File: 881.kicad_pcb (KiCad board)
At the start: 2 copper layers, 38 x 105 mm, 0 parts

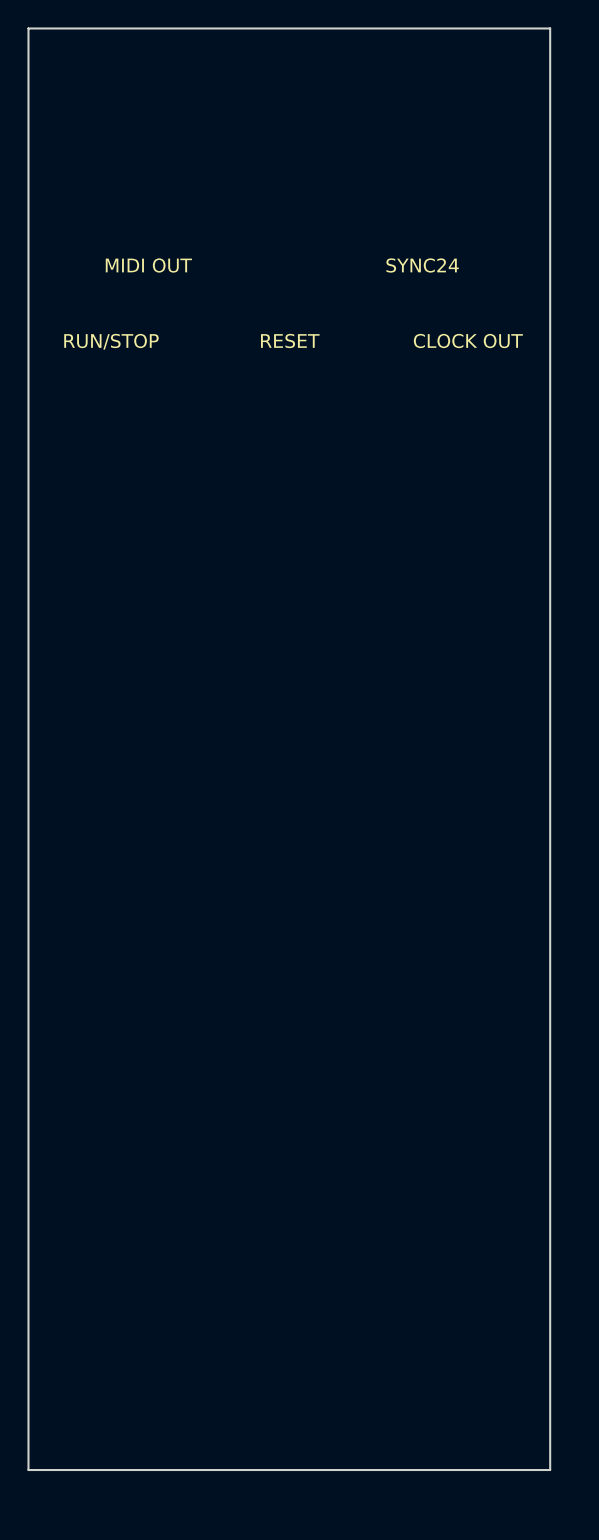
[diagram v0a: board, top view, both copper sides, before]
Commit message: first route
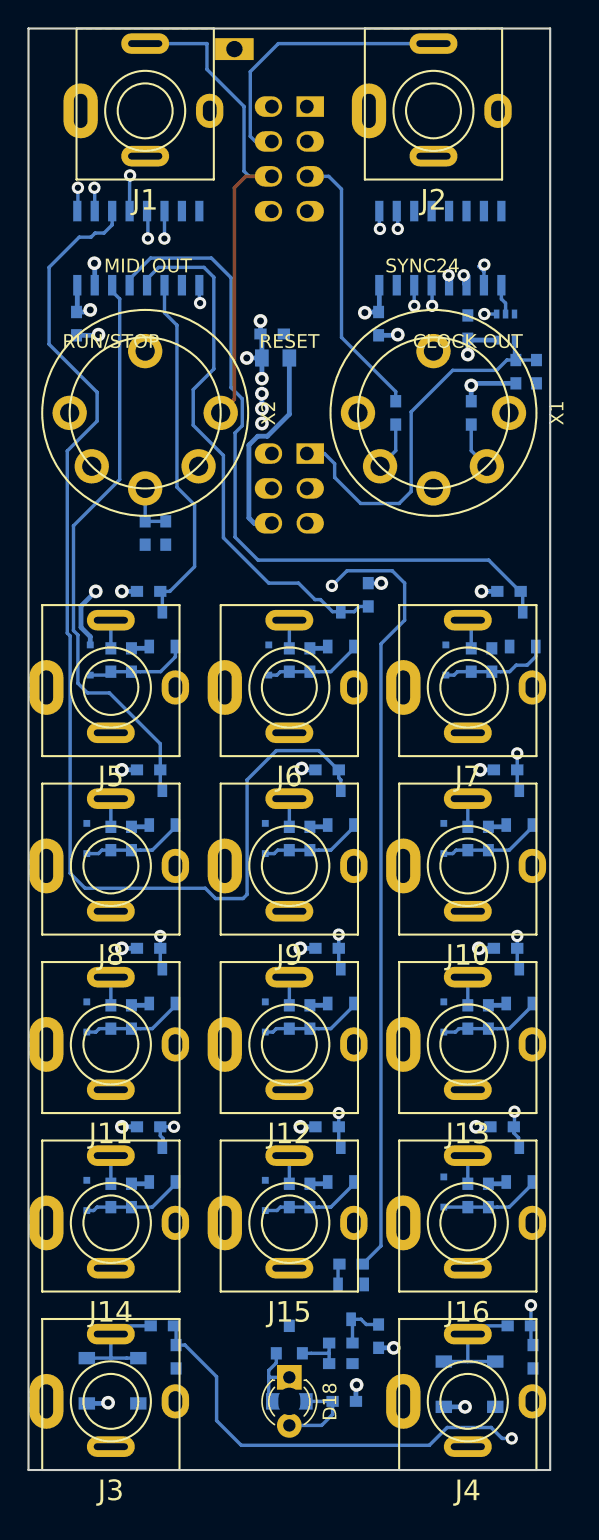
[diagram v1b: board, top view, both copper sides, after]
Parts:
- added C1: 0.01µ, MyModules:SM0603-C-MURATA, B.Cu at (121.5, 91.8)
- added C15: 1µ, Capacitors_SMD:C_0805, B.Cu at (129.5, 79.0)
- added C19: 0.1µ, MyModules:SM0603-C-MURATA, B.Cu at (129.2, 77.2)
- added C2: 0.1µ, MyModules:SM0603-C-MURATA, B.Cu at (115.0, 76.5)
- added C20: 0.1µ, MyModules:SM0603-C-MURATA, B.Cu at (143.5, 76.8)
- added C3: 0.1µ, MyModules:SM0603-C-MURATA, B.Cu at (137.0, 76.5)
- added C4: 1n, MyModules:SM0603-C-MURATA, B.Cu at (134.2, 152.2)
- added D1: B5819W, Diodes_SMD:D_SOD-123, B.Cu at (115.8, 153.5)
- added D10: 1N4148, Diodes_SMD:D_SOD-323F, B.Cu at (141.8, 114.0)
- added D11: 1N4148, Diodes_SMD:D_SOD-323F, B.Cu at (115.8, 127.0)
- added D12: 1N4148, Diodes_SMD:D_SOD-323F, B.Cu at (128.8, 127.0)
- added D13: 1N4148, Diodes_SMD:D_SOD-323F, B.Cu at (141.8, 127.0)
- added D14: 1N4148, Diodes_SMD:D_SOD-323F, B.Cu at (115.8, 140.0)
- added D15: 1N4148, Diodes_SMD:D_SOD-323F, B.Cu at (128.8, 140.0)
- added D16: 1N4148, Diodes_SMD:D_SOD-323F, B.Cu at (141.8, 139.8)
- added D17: LED, LEDs:LED_0805, B.Cu at (130.5, 155.0)
- added D18: LED, LEDs:LED_D3.0mm, F.Cu at (130.5, 153.8)
- added D2: B5819W, Diodes_SMD:D_SOD-123, B.Cu at (119.5, 153.5)
- added D3: B5819W, Diodes_SMD:D_SOD-123, B.Cu at (141.8, 153.8)
- added D4: B5819W, Diodes_SMD:D_SOD-123, B.Cu at (145.5, 153.8)
- added D5: 1N4148, Diodes_SMD:D_SOD-323F, B.Cu at (116.0, 101.0)
- added D6: 1N4148, Diodes_SMD:D_SOD-323F, B.Cu at (129.0, 101.0)
- added D7: 1N4148, Diodes_SMD:D_SOD-323F, B.Cu at (141.9, 101.0)
- added D8: 1N4148, Diodes_SMD:D_SOD-323F, B.Cu at (115.8, 114.0)
- added D9: 1N4148, Diodes_SMD:D_SOD-323F, B.Cu at (128.8, 114.0)
- added ISP1: CONN_02X03, w_conn_strip:vasch_strip_3x2, B.Cu at (130.5, 88.5)
- added J1: RUN/STOP, MyModules:PJ-301B-JACK-SLOTS, F.Cu at (120.0, 61.0)
- added J10: RS IN, MyModules:PJ-301B-JACK-SLOTS, F.Cu at (143.5, 116.0)
- added J11: CP IN, MyModules:PJ-301B-JACK-SLOTS, F.Cu at (117.5, 129.0)
- added J12: MA IN, MyModules:PJ-301B-JACK-SLOTS, F.Cu at (130.5, 129.0)
- added J13: CB IN, MyModules:PJ-301B-JACK-SLOTS, F.Cu at (143.5, 129.0)
- added J14: CY IN, MyModules:PJ-301B-JACK-SLOTS, F.Cu at (117.5, 142.0)
- added J15: OH IN, MyModules:PJ-301B-JACK-SLOTS, F.Cu at (130.5, 142.0)
- added J16: CH IN, MyModules:PJ-301B-JACK-SLOTS, F.Cu at (143.5, 142.0)
- added J2: SYNC24 CLK, MyModules:PJ-301B-JACK-SLOTS, F.Cu at (141.0, 61.0)
- added J3: ASSIGN 1, MyModules:PJ-301B-JACK-SLOTS, F.Cu at (117.5, 155.0)
- added J4: ASSIGN 2, MyModules:PJ-301B-JACK-SLOTS, F.Cu at (143.5, 155.0)
- added J5: BD IN, MyModules:PJ-301B-JACK-SLOTS, F.Cu at (117.5, 103.0)
- added J6: SD IN, MyModules:PJ-301B-JACK-SLOTS, F.Cu at (130.5, 103.0)
- added J7: LT IN, MyModules:PJ-301B-JACK-SLOTS, F.Cu at (143.5, 103.0)
- added J8: MT IN, MyModules:PJ-301B-JACK-SLOTS, F.Cu at (117.5, 116.0)
- added J9: HT IN, MyModules:PJ-301B-JACK-SLOTS, F.Cu at (130.5, 116.0)
- added P1: CONN_02X03, w_conn_strip:vasch_strip_4x2, B.Cu at (130.5, 64.5)
- added Q1: MMBT3904, MyModules:SOT23-132-JRL, B.Cu at (121.2, 98.8)
- added Q10: MMBT3904, MyModules:SOT23-132-JRL, B.Cu at (121.2, 137.8)
- added Q11: MMBT3904, MyModules:SOT23-132-JRL, B.Cu at (134.2, 137.8)
- added Q12: MMBT3904, MyModules:SOT23-132-JRL, B.Cu at (147.2, 137.8)
- added Q13: MMBT3904, MyModules:SOT23-132-JRL, B.Cu at (135.0, 147.8)
- added Q14: MMBT3906, SOT-23, B.Cu at (130.5, 150.5)
- added Q2: MMBT3904, MyModules:SOT23-132-JRL, B.Cu at (134.2, 98.8)
- added Q3: MMBT3904, MyModules:SOT23-132-JRL, B.Cu at (147.5, 98.8)
- added Q4: MMBT3904, MyModules:SOT23-132-JRL, B.Cu at (121.2, 111.8)
- added Q5: MMBT3904, MyModules:SOT23-132-JRL, B.Cu at (134.2, 111.8)
- added Q6: MMBT3904, MyModules:SOT23-132-JRL, B.Cu at (147.2, 111.8)
- added Q7: MMBT3904, MyModules:SOT23-132-JRL, B.Cu at (121.2, 124.8)
- added Q8: MMBT3904, MyModules:SOT23-132-JRL, B.Cu at (134.2, 124.8)
- added Q9: MMBT3904, MyModules:SOT23-132-JRL, B.Cu at (147.2, 124.8)
- added R1: 220, MyModules:SM0603-R-YAGEO, B.Cu at (138.2, 83.0)
- added R10: 100K, MyModules:SM0603-R-YAGEO, B.Cu at (119.0, 101.0)
- added R11: 100K, MyModules:SM0603-R-YAGEO, B.Cu at (132.0, 101.0)
- added R12: 100K, MyModules:SM0603-R-YAGEO, B.Cu at (145.2, 101.0)
- added R13: 100K, MyModules:SM0603-R-YAGEO, B.Cu at (119.0, 114.0)
- added R14: 10K, MyModules:SM0603-R-YAGEO, B.Cu at (120.2, 96.0)
- added R15: 10K, MyModules:SM0603-R-YAGEO, B.Cu at (136.2, 96.2)
- added R16: 10K, MyModules:SM0603-R-YAGEO, B.Cu at (146.5, 96.0)
- added R17: 10K, MyModules:SM0603-R-YAGEO, B.Cu at (120.2, 109.0)
- added R18: 100K, MyModules:SM0603-R-YAGEO, B.Cu at (130.5, 114.0)
- added R19: 100K, MyModules:SM0603-R-YAGEO, B.Cu at (143.5, 114.0)
- added R2: 22, MyModules:SM0603-R-YAGEO, B.Cu at (120.0, 91.8)
- added R20: 100K, MyModules:SM0603-R-YAGEO, B.Cu at (117.5, 127.0)
- added R21: 100K, MyModules:SM0603-R-YAGEO, B.Cu at (130.5, 127.0)
- added R22: 100K, MyModules:SM0603-R-YAGEO, B.Cu at (132.0, 114.0)
- added R23: 100K, MyModules:SM0603-R-YAGEO, B.Cu at (145.0, 114.0)
- added R24: 100K, MyModules:SM0603-R-YAGEO, B.Cu at (119.0, 127.0)
- added R25: 100K, MyModules:SM0603-R-YAGEO, B.Cu at (132.0, 127.0)
- added R26: 10K, MyModules:SM0603-R-YAGEO, B.Cu at (133.2, 109.0)
- added R27: 10K, MyModules:SM0603-R-YAGEO, B.Cu at (146.2, 109.0)
- added R28: 10K, MyModules:SM0603-R-YAGEO, B.Cu at (120.2, 122.0)
- added R29: 10K, MyModules:SM0603-R-YAGEO, B.Cu at (133.2, 122.0)
- added R3: 220, MyModules:SM0603-R-YAGEO, B.Cu at (143.8, 83.0)
- added R30: 100K, MyModules:SM0603-R-YAGEO, B.Cu at (143.5, 127.0)
- added R31: 100K, MyModules:SM0603-R-YAGEO, B.Cu at (117.5, 140.0)
- added R32: 100K, MyModules:SM0603-R-YAGEO, B.Cu at (130.5, 140.0)
- added R33: 100K, MyModules:SM0603-R-YAGEO, B.Cu at (143.5, 140.0)
- added R34: 100K, MyModules:SM0603-R-YAGEO, B.Cu at (145.0, 127.0)
- added R35: 100K, MyModules:SM0603-R-YAGEO, B.Cu at (119.0, 140.0)
- added R36: 100K, MyModules:SM0603-R-YAGEO, B.Cu at (132.0, 140.0)
- added R37: 100K, MyModules:SM0603-R-YAGEO, B.Cu at (145.0, 140.0)
- added R38: 10K, MyModules:SM0603-R-YAGEO, B.Cu at (146.2, 122.0)
- added R39: 10K, MyModules:SM0603-R-YAGEO, B.Cu at (120.2, 135.0)
- added R4: 1K, MyModules:SM0603-R-YAGEO, B.Cu at (121.2, 149.5)
- added R40: 10K, MyModules:SM0603-R-YAGEO, B.Cu at (133.2, 135.0)
- added R41: 10K, MyModules:SM0603-R-YAGEO, B.Cu at (146.0, 135.0)
- added R42: 47K, MyModules:SM0603-R-YAGEO, B.Cu at (122.2, 151.8)
- added R43: 100K, MyModules:SM0603-R-YAGEO, B.Cu at (148.2, 151.8)
- added R44: 47K, MyModules:SM0603-R-YAGEO, B.Cu at (147.0, 80.0)
- added R45: 47K, MyModules:SM0603-R-YAGEO, B.Cu at (148.5, 80.0)
- added R46: 100K, MyModules:SM0603-R-YAGEO, B.Cu at (135.0, 145.0)
- added R47: 1K, MyModules:SM0603-R-YAGEO, B.Cu at (137.0, 150.2)
- added R48: 10K, MyModules:SM0603-R-YAGEO, B.Cu at (134.2, 150.8)
- added R49: 1K, MyModules:SM0603-R-YAGEO, B.Cu at (134.5, 155.0)
- added R5: 1K, MyModules:SM0603-R-YAGEO, B.Cu at (147.2, 149.5)
- added R6: 100K, MyModules:SM0603-R-YAGEO, B.Cu at (117.5, 101.0)
- added R7: 100K, MyModules:SM0603-R-YAGEO, B.Cu at (130.5, 101.0)
- added R8: 100K, MyModules:SM0603-R-YAGEO, B.Cu at (143.8, 101.0)
- added R9: 100K, MyModules:SM0603-R-YAGEO, B.Cu at (117.5, 114.0)
- added TP2: CONN_1, MyModules:TEST_POINT_LOOP_4592, B.Cu at (126.5, 56.5)
- added U1: 74HC165, Housings_SOIC:SOIC-16_3.9x9.9mm_Pitch1.27mm, B.Cu at (119.5, 71.0)
- added U2: 74HC165, Housings_SOIC:SOIC-16_3.9x9.9mm_Pitch1.27mm, B.Cu at (141.5, 71.0)
- added U7: 74AHCT1G125GW, TO_SOT_Packages_SMD:SOT-353_SC-70-5, B.Cu at (146.2, 76.8)
- added X1: MIDI OUT, MyModules:SD-50BV-5DIN, F.Cu at (141.0, 83.0)
- added X2: SYNC24, MyModules:SD-50BV-5DIN, F.Cu at (120.0, 83.0)
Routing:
- net DIN_RESET: track 0.00 -> 143.3 mm, vias 0 -> 1
- net ISP_SCK: track 0.00 -> 117.2 mm, vias 0 -> 3
- net DIN_FILL: track 0.00 -> 109.5 mm, vias 0 -> 1
- net /HT: track 0.00 -> 85.3 mm
- net /CY: track 0.00 -> 77.1 mm, vias 0 -> 2
- net /RS: track 0.00 -> 75.7 mm, vias 0 -> 2
- net /CH: track 0.00 -> 72.6 mm, vias 0 -> 2
- net /OH: track 0.00 -> 67.1 mm, vias 0 -> 2
- net DIN_RUN_STOP: track 0.00 -> 67.0 mm, vias 0 -> 1
- net /MA: track 0.00 -> 60.5 mm, vias 0 -> 2
- net /CP: track 0.00 -> 56.4 mm, vias 0 -> 2
- net /CB: track 0.00 -> 54.5 mm, vias 0 -> 2
- net DIN_TEMPO_CLK: track 0.00 -> 53.4 mm
- net /LT: track 0.00 -> 52.5 mm
- net ISP_MOSI: track 0.00 -> 47.2 mm, vias 0 -> 2
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- added copper zone on In2.Cu, net +5V
- added copper zone on B.Cu, net GNDD
- added copper zone on F.Cu, net GNDD
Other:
- copper layers 2 -> 4
- net class Default: via_dia 0.8 -> 0.9; via_drill 0.4 -> 0.45
- net class POWER: via_dia 0.9 -> 1; via_drill 0.45 -> 0.5
